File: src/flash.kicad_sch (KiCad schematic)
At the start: 17 parts, among them J2 Micro_SD_Card_Det1, U1 ECP5U_12_CABGA256, U11 W25Q128JVS

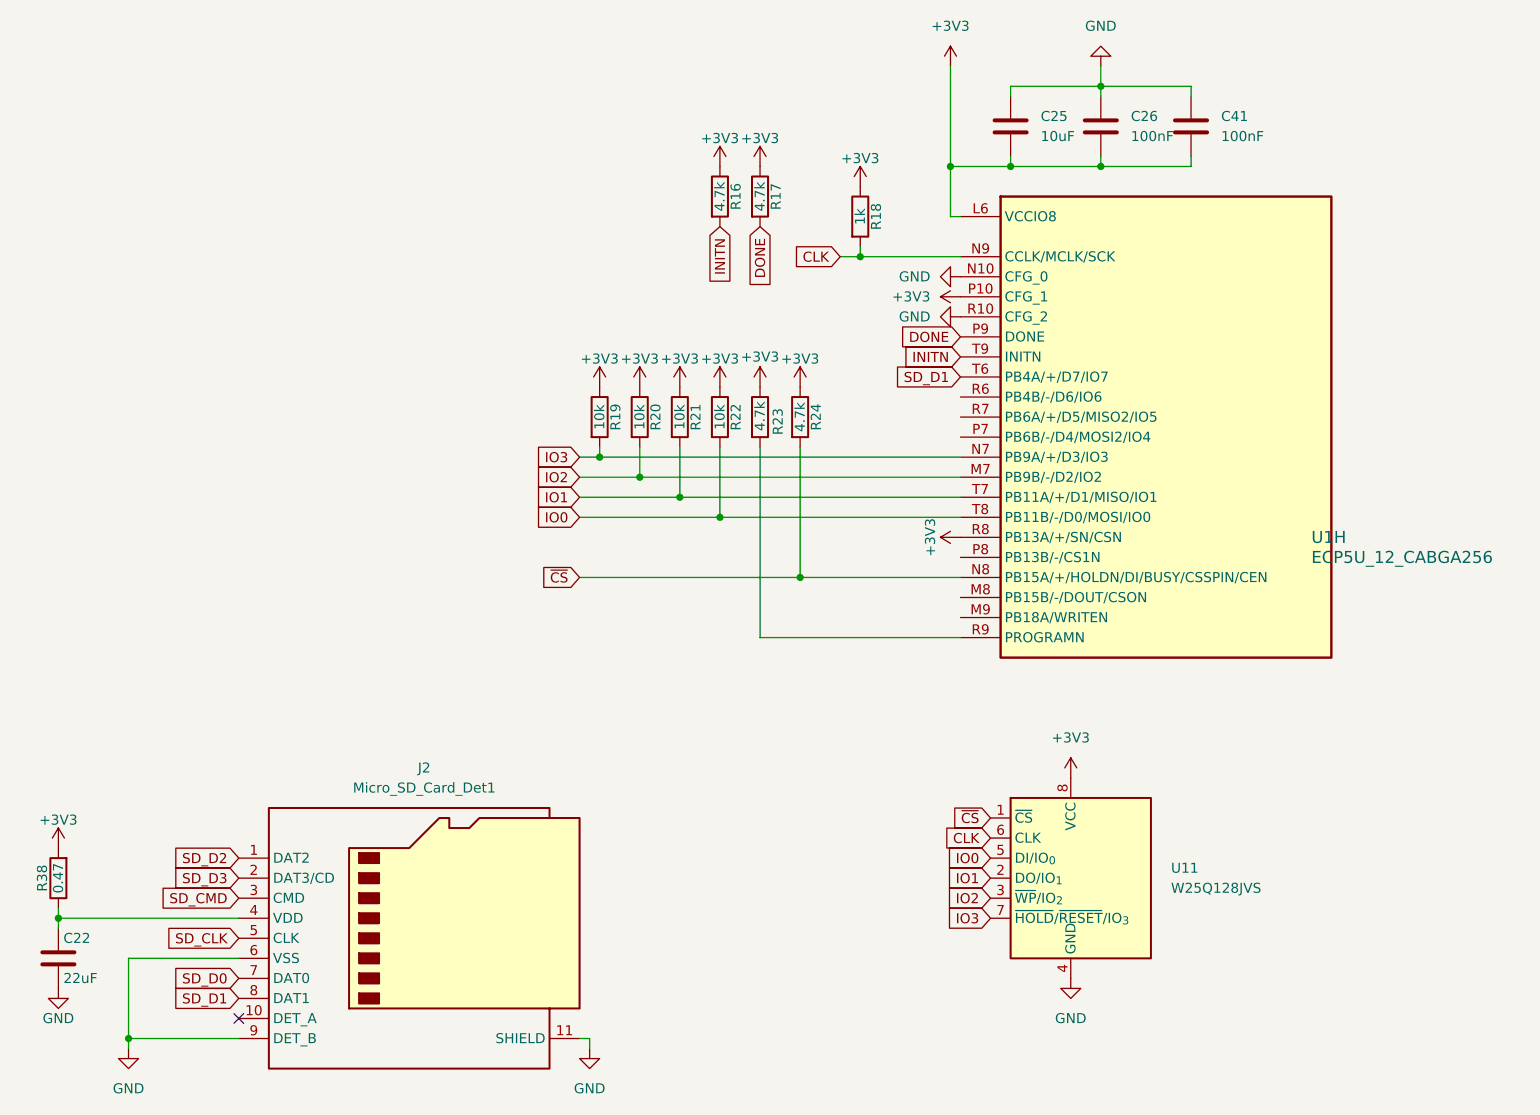
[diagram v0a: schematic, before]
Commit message: Rev 2
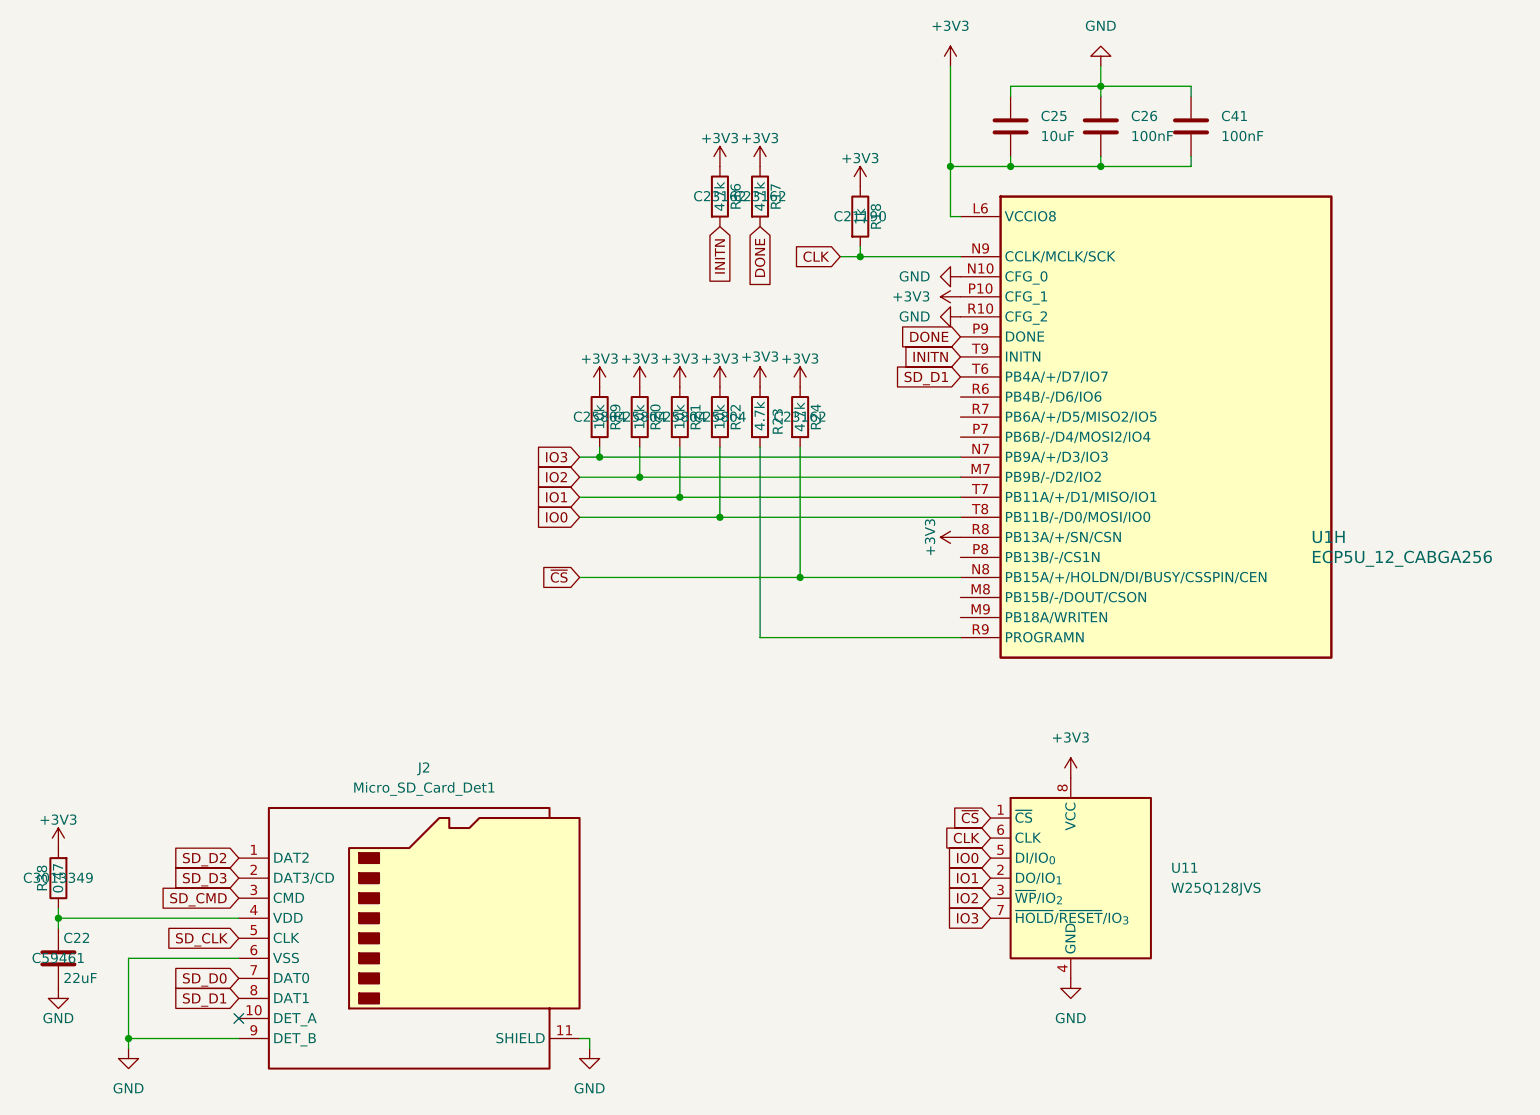
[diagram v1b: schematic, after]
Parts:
- C22: LCSC Part (none) -> C59461; MNF1_URL www.yageo.com -> (none); MPN CC0805ZKY5V5BB226 -> (none)
- C25: LCSC Part (none) -> C19702
- C26, C41: LCSC Part (none) -> C1525
- R16, R17, R24: LCSC Part (none) -> C23162; MNF1_URL www.yageo.com -> (none); MPN AC0603FR-104K7L -> (none)
- R18: LCSC Part (none) -> C21190
- R19: Digikey 311-10KLMCT-ND -> (none); Koncar FR013 -> (none); LCSC C15401 -> (none); LCSC Part (none) -> C25804; MNF1_URL www.yageo.com -> (none); MPN RC0603FR-0710KL -> (none); Mouser 603-RC0603FR-0710KL -> (none); Newark 94X1379 -> (none)
- R20, R21, R22: LCSC Part (none) -> C25804
- R23: LCSC Part (none) -> C23162; MPN RC0402JR-075K1L -> (none); Manufacturer Yageo -> (none); Manufacturer2 UNI-ROYAL(Uniroyal Elec) -> (none)
- R38: Digikey 73L2R47JCT-ND -> (none); Koncar FR001 -> (none); LCSC C158884 -> (none); LCSC Part (none) -> C3013349; MFG1 CTS -> (none); MNF1_URL www.ctscorp.com -> (none); MPN 73L2R47J -> (none); Mouser 774-73L2R47J -> (none); Newark 32K1357 -> (none)
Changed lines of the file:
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@@
+			)
+		)
+		(property "LCSC Part" "C25804"
+			(at 114.3 82.55 0)
+			(effects
+				(font
+					(size 1.27 1.27)
+				)
 			)
 		)
@@
 			)
 		)
+		(property "LCSC Part" "C25804"
+			(at 119.38 82.55 0)
+			(effects
+				(font
+					(size 1.27 1.27)
+				)
+			)
+		)
 		(pin "1"
 		)
@@
 			)
 		)
+		(property "LCSC Part" "C21190"
+			(at 137.16 57.15 0)
+			(effects
+				(font
+					(size 1.27 1.27)
+				)
+			)
+		)
 		(pin "1"
 		)
@@
 			)
 		)
-		(property "MNF1_URL" "www.yageo.com"
-			(at 129.54 82.55 90)
-			(effects
-				(font
-					(size 1.27 1.27)
-				)
-				(hide yes)
-			)
-		)
-		(property "MPN" "AC0603FR-104K7L"
-			(at 129.54 82.55 90)
-			(effects
-				(font
-					(size 1.27 1.27)
-				)
-				(hide yes)
+		(property "LCSC Part" "C23162"
+			(at 129.54 82.55 0)
+			(effects
+				(font
+					(size 1.27 1.27)
+				)
 			)
 		)
@@
 			)
 		)
+		(property "LCSC Part" "C25804"
+			(at 109.22 82.55 0)
+			(effects
+				(font
+					(size 1.27 1.27)
+				)
+			)
+		)
 		(pin "1"
 		)
@@
 			)
 		)
-		(property "MFG1" "CTS"
-			(at 35.56 140.97 90)
-			(effects
-				(font
-					(size 1.27 1.27)
-				)
-				(hide yes)
-			)
-		)
-		(property "MNF1_URL" "www.ctscorp.com"
-			(at 35.56 140.97 90)
-			(effects
-				(font
-					(size 1.27 1.27)
-				)
-				(hide yes)
-			)
-		)
-		(property "MPN" "73L2R47J"
-			(at 35.56 140.97 90)
-			(effects
-				(font
-					(size 1.27 1.27)
-				)
-				(hide yes)
-			)
-		)
-		(property "Mouser" "774-73L2R47J"
-			(at 35.56 140.97 90)
-			(effects
-				(font
-					(size 1.27 1.27)
-				)
-				(hide yes)
-			)
-		)
-		(property "Digikey" "73L2R47JCT-ND"
-			(at 35.56 140.97 90)
-			(effects
-				(font
-					(size 1.27 1.27)
-				)
-				(hide yes)
-			)
-		)
-		(property "Newark" "32K1357"
-			(at 35.56 140.97 90)
-			(effects
-				(font
-					(size 1.27 1.27)
-				)
-				(hide yes)
-			)
-		)
-		(property "LCSC" "C158884"
-			(at 35.56 140.97 90)
-			(effects
-				(font
-					(size 1.27 1.27)
-				)
-				(hide yes)
-			)
-		)
-		(property "Koncar" "FR001"
-			(at 35.56 140.97 90)
-			(effects
-				(font
-					(size 1.27 1.27)
-				)
-				(hide yes)
+		(property "LCSC Part" "C3013349"
+			(at 35.56 140.97 0)
+			(effects
+				(font
+					(size 1.27 1.27)
+				)
 			)
 		)
@@
 			)
 		)
-		(property "LCSC Part" ""
+		(property "LCSC Part" "C19702"
 			(at 156.21 45.72 0)
 			(effects
@@
 			)
 		)
-		(property "MNF1_URL" "www.yageo.com"
-			(at 119.38 54.61 90)
-			(effects
-				(font
-					(size 1.27 1.27)
-				)
-				(hide yes)
-			)
-		)
-		(property "MPN" "AC0603FR-104K7L"
-			(at 119.38 54.61 90)
-			(effects
-				(font
-					(size 1.27 1.27)
-				)
-				(hide yes)
+		(property "LCSC Part" "C23162"
+			(at 119.38 54.61 0)
+			(effects
+				(font
+					(size 1.27 1.27)
+				)
 			)
 		)
@@
 			)
 		)
-		(property "MNF1_URL" "www.yageo.com"
-			(at 124.46 54.61 90)
-			(effects
-				(font
-					(size 1.27 1.27)
-				)
-				(hide yes)
-			)
-		)
-		(property "MPN" "AC0603FR-104K7L"
-			(at 124.46 54.61 90)
-			(effects
-				(font
-					(size 1.27 1.27)
-				)
-				(hide yes)
+		(property "LCSC Part" "C23162"
+			(at 124.46 54.61 0)
+			(effects
+				(font
+					(size 1.27 1.27)
+				)
 			)
 		)
@@
 			)
 		)
-		(property "LCSC Part" ""
+		(property "LCSC Part" "C1525"
 			(at 179.07 45.72 0)
 			(effects
@@
 			)
 		)
-		(property "MNF1_URL" "www.yageo.com"
+		(property "LCSC Part" "C59461"
 			(at 35.56 151.13 0)
 			(effects
@@
 					(size 1.27 1.27)
 				)
-				(hide yes)
-			)
-		)
-		(property "MPN" "CC0805ZKY5V5BB226 "
-			(at 35.56 151.13 0)
-			(effects
-				(font
-					(size 1.27 1.27)
-				)
-				(hide yes)
 			)
 		)
@@
 			)
 		)
-		(property "MNF1_URL" "www.yageo.com"
-			(at 104.14 82.55 90)
-			(effects
-				(font
-					(size 1.27 1.27)
-				)
-				(hide yes)
-			)
-		)
-		(property "MPN" "RC0603FR-0710KL"
-			(at 104.14 82.55 90)
-			(effects
-				(font
-					(size 1.27 1.27)
-				)
-				(hide yes)
-			)
-		)
-		(property "Mouser" "603-RC0603FR-0710KL"
-			(at 104.14 82.55 90)
-			(effects
-				(font
-					(size 1.27 1.27)
-				)
-				(hide yes)
-			)
-		)
-		(property "Digikey" "311-10KLMCT-ND"
-			(at 104.14 82.55 90)
-			(effects
-				(font
-					(size 1.27 1.27)
-				)
-				(hide yes)
-			)
-		)
-		(property "Newark" "94X1379"
-			(at 104.14 82.55 90)
-			(effects
-				(font
-					(size 1.27 1.27)
-				)
-				(hide yes)
-			)
-		)
-		(property "LCSC" "C15401"
-			(at 104.14 82.55 90)
-			(effects
-				(font
-					(size 1.27 1.27)
-				)
-				(hide yes)
-			)
-		)
-		(property "Koncar" "FR013"
-			(at 104.14 82.55 90)
-			(effects
-				(font
-					(size 1.27 1.27)
-				)
-				(hide yes)
+		(property "LCSC Part" "C25804"
+			(at 104.14 82.55 0)
+			(effects
+				(font
+					(size 1.27 1.27)
+				)
 			)
 		)
@@
 			)
 		)
-		(property "LCSC Part" ""
+		(property "LCSC Part" "C1525"
 			(at 167.64 45.72 0)
 			(effects
@@
 			)
 		)
-		(property "DNP" ""
-			(at 125.73 83.82 0)
-			(effects
-				(font
-					(size 1.27 1.27)
-				)
-				(justify left top)
-			)
-		)
-		(property "MPN" "RC0402JR-075K1L\n"
+		(property "LCSC Part" "C23162"
 			(at 124.46 82.55 0)
 			(effects
-				(font
-					(size 1.27 1.27)
-				)
-				(hide yes)
-			)
-		)
-		(property "Manufacturer" "Yageo"
-			(at 124.46 82.55 0)
-			(effects
-				(font
-					(size 1.27 1.27)
-				)
-				(hide yes)
-			)
-		)
-		(property "Manufacturer2" "UNI-ROYAL(Uniroyal Elec)"
-			(at 124.46 82.55 0)
-			(effects
-				(font
-					(size 1.27 1.27)
-				)
-				(hide yes)
-			)
-		)
-		(property "LCSC Part" ""
-			(at 124.46 82.55 0)
-			(effects

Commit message: Tidy project
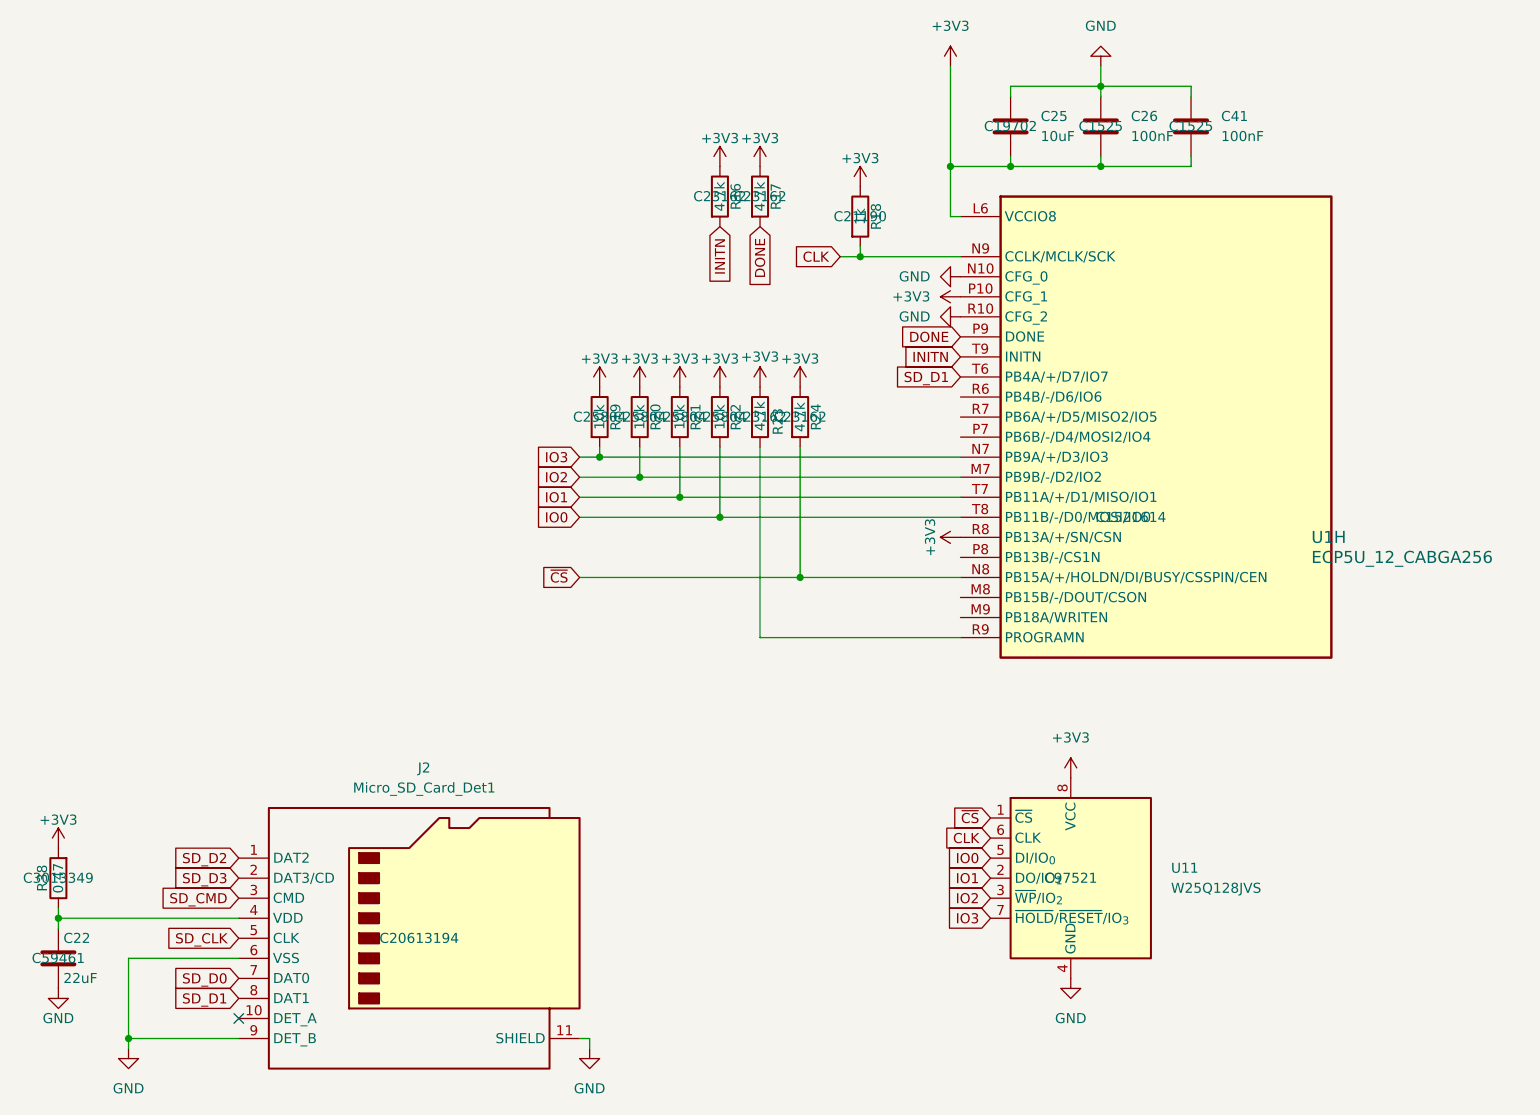
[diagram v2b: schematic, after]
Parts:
- C22: JLCPCB Part # (none) -> C59461; LCSC Part C59461 -> (none)
- C25: JLCPCB Part # (none) -> C19702; LCSC Part C19702 -> (none)
- C26, C41: JLCPCB Part # (none) -> C1525; LCSC Part C1525 -> (none)
- J2: JLCPCB Part # (none) -> C20613194; LCSC Part C20613194 -> (none)
- R16, R17, R23, R24: JLCPCB Part # (none) -> C23162; LCSC Part C23162 -> (none)
- R18: JLCPCB Part # (none) -> C21190; LCSC Part C21190 -> (none)
- R19, R20, R21, R22: JLCPCB Part # (none) -> C25804; LCSC Part C25804 -> (none)
- R38: JLCPCB Part # (none) -> C3013349; LCSC Part C3013349 -> (none)
- U1: JLCPCB Part # (none) -> C1521614; LCSC Part C1521614 -> (none)
- U11: JLCPCB Part # (none) -> C97521; LCSC Part C97521 -> (none)
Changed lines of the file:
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@@
 			)
 		)
-		(property "LCSC Part" "C25804"
+		(property "JLCPCB Part #" "C25804"
 			(at 114.3 82.55 0)
 			(effects
@@
 			)
 		)
-		(property "LCSC Part" "C25804"
+		(property "JLCPCB Part #" "C25804"
 			(at 119.38 82.55 0)
 			(effects
@@
 			)
 		)
-		(property "LCSC Part" "C21190"
+		(property "JLCPCB Part #" "C21190"
 			(at 137.16 57.15 0)
 			(effects
@@
 			)
 		)
-		(property "LCSC Part" "C23162"
+		(property "JLCPCB Part #" "C23162"
 			(at 129.54 82.55 0)
 			(effects
@@
 			)
 		)
-		(property "LCSC Part" "C25804"
+		(property "JLCPCB Part #" "C25804"
 			(at 109.22 82.55 0)
 			(effects
@@
 			)
 		)
-		(property "LCSC Part" "C3013349"
+		(property "JLCPCB Part #" "C3013349"
 			(at 35.56 140.97 0)
 			(effects
@@
 			)
 		)
-		(property "LCSC Part" "C20613194"
+		(property "JLCPCB Part #" "C20613194"
 			(at 81.28 148.59 0)
 			(effects
@@
 					(size 1.27 1.27)
 				)
-				(hide yes)
 			)
 		)
@@
 			)
 		)
-		(property "LCSC Part" "C19702"
+		(property "JLCPCB Part #" "C19702"
 			(at 156.21 45.72 0)
 			(effects
@@
 					(size 1.27 1.27)
 				)
-				(hide yes)
 			)
 		)
@@
 			)
 		)
-		(property "LCSC Part" "C23162"
+		(property "JLCPCB Part #" "C23162"
 			(at 119.38 54.61 0)
 			(effects
@@
 			)
 		)
-		(property "LCSC Part" "C23162"
+		(property "JLCPCB Part #" "C23162"
 			(at 124.46 54.61 0)
 			(effects
@@
 			)
 		)
-		(property "LCSC Part" " C1521614"
+		(property "JLCPCB Part #" " C1521614"
 			(at 171.45 95.25 0)
 			(effects
@@
 					(size 1.27 1.27)
 				)
-				(hide yes)
 			)
 		)
@@
 			)
 		)
-		(property "LCSC Part" "C1525"
+		(property "JLCPCB Part #" "C1525"
 			(at 179.07 45.72 0)
 			(effects
@@
 					(size 1.27 1.27)
 				)
-				(hide yes)
 			)
 		)
@@
 			)
 		)
-		(property "LCSC Part" " C97521"
+		(property "JLCPCB Part #" " C97521"
 			(at 163.83 140.97 0)
 			(effects
@@
 					(size 1.27 1.27)
 				)
-				(hide yes)
 			)
 		)
@@
 			)
 		)
-		(property "LCSC Part" "C59461"
+		(property "JLCPCB Part #" "C59461"
 			(at 35.56 151.13 0)
 			(effects
@@
 			)
 		)
-		(property "LCSC Part" "C25804"
+		(property "JLCPCB Part #" "C25804"
 			(at 104.14 82.55 0)
 			(effects
@@
 			)
 		)
-		(property "LCSC Part" "C1525"
+		(property "JLCPCB Part #" "C1525"
 			(at 167.64 45.72 0)
 			(effects
@@
 					(size 1.27 1.27)
 				)
-				(hide yes)
 			)
 		)
@@
 			)
 		)
-		(property "LCSC Part" "C23162"
+		(property "JLCPCB Part #" "C23162"
 			(at 124.46 82.55 0)
 			(effects
@@
 					(size 1.27 1.27)
 				)
-				(hide yes)
-			)
-		)
+			)
+		)
